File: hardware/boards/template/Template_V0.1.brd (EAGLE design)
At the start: 44 x 44 mm, 2 parts

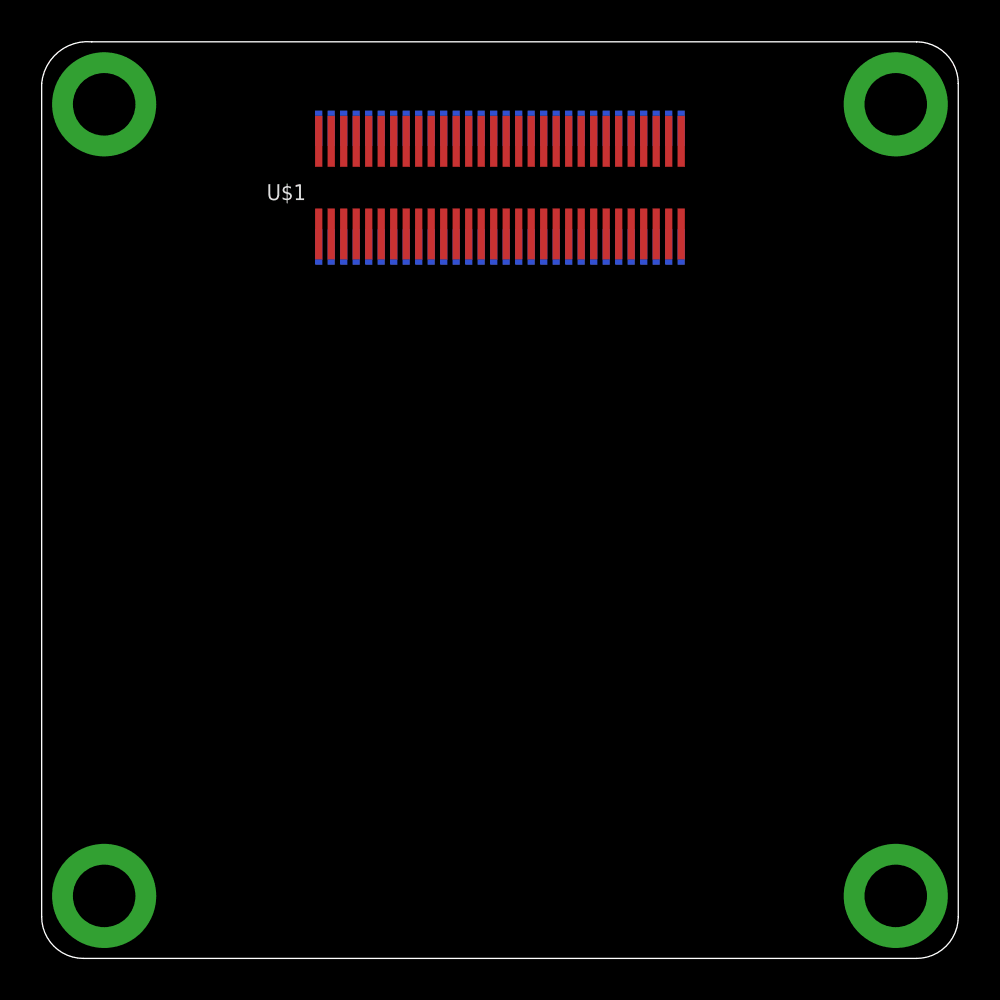
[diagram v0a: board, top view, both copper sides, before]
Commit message: Updating template, wip
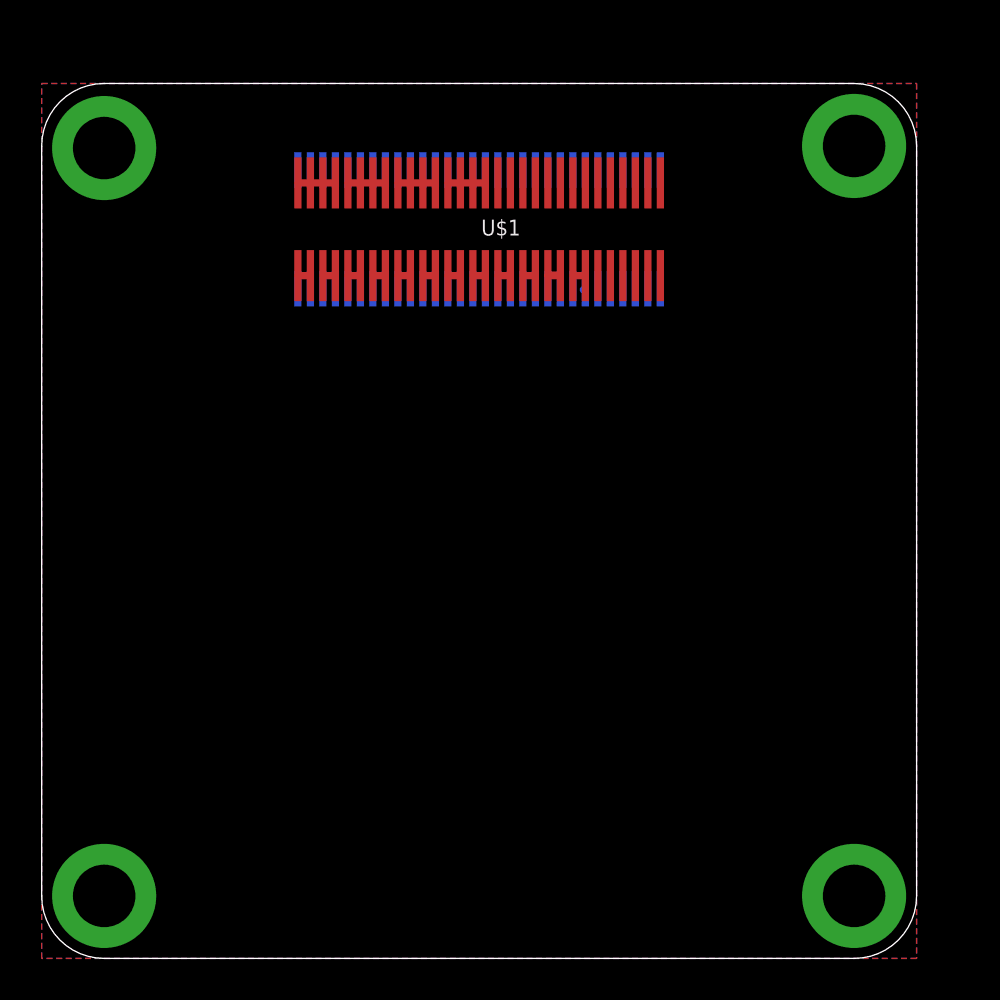
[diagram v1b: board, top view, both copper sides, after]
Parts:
- moved U$1 2.24 mm to (21.0, 35.0)
- moved U$3 2.24 mm to (21.0, 35.0)
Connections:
- removed net +3.3V_SW2: U$1.P$10, U$3.P$51
- removed net +3.3V_SW3: U$1.P$11, U$3.P$50
- removed net VBUS_1: U$1.P$53
- removed net VBUS_2: U$1.P$54
- removed net VBUS_3: U$1.P$55
- removed net VBUS_SW1: U$1.P$6, U$3.P$55
- removed net VBUS_SW2: U$1.P$7, U$3.P$54
- removed net VBUS_SW3: U$1.P$8, U$3.P$53
- new net +3V3_BUS: U$1.P$57, U$1.P$58, U$1.P$59, U$1.P$60
- new net +3V3_SW2: U$1.P$5, U$1.P$6, U$3.P$55, U$3.P$56
- new net +3V3_SW3: U$1.P$10, U$1.P$9, U$3.P$51, U$3.P$52
- new net /RST: U$1.P$27, U$3.P$34
- new net /SS/GPIO2: U$1.P$34
- new net 33-GND: U$3.P$3
- new net 37-GND: U$3.P$7
- new net 41-GND: U$3.P$11
- new net 44-GND: U$3.P$14
- new net 46-GND: U$3.P$16
- new net 48-GND: U$3.P$18
- new net 49-GND: U$3.P$19
- new net 57-GND: U$3.P$27
- new net 59-GND: U$3.P$29
- new net BATV_BUS: U$1.P$49, U$1.P$50, U$1.P$51, U$1.P$52
- new net BATV_SW1: U$1.P$13, U$1.P$14, U$3.P$47, U$3.P$48
- new net BATV_SW2: U$1.P$17, U$1.P$18, U$3.P$43, U$3.P$44
- new net BATV_SW3: U$1.P$21, U$1.P$22, U$3.P$39, U$3.P$40
- new net GPIO0: U$1.P$25, U$3.P$36
- new net GPIO1: U$1.P$26, U$3.P$35
- new net GPIO11: U$1.P$43
- new net GPIO12: U$1.P$44
- new net GPIO3: U$1.P$35
- new net GPIO4: U$1.P$36
- new net GPIO5: U$1.P$37
- new net GPIO6: U$1.P$38
- new net GPIO7: U$1.P$39
- new net GPIO8: U$1.P$40
- new net GPIO9: U$1.P$41
- new net MISO: U$1.P$32
- new net MOSI: U$1.P$31
- new net RTN_+3V3: U$1.P$53, U$1.P$54, U$1.P$55, U$1.P$56
- new net RTN_+3V3_SW1: U$1.P$3, U$1.P$4, U$3.P$57, U$3.P$58
- new net RTN_+3V3_SW2: U$1.P$7, U$1.P$8, U$3.P$53, U$3.P$54
- new net RTN_+3V3_SW3: U$1.P$11, U$1.P$12, U$3.P$49, U$3.P$50
- new net RTN_BATV: U$1.P$45, U$1.P$46, U$1.P$47, U$1.P$48
- new net RTN_BATV_SW1: U$1.P$15, U$1.P$16, U$3.P$45, U$3.P$46
- new net RTN_BATV_SW2: U$1.P$19, U$1.P$20, U$3.P$41, U$3.P$42
- new net RTN_BATV_SW3: U$1.P$23, U$1.P$24, U$3.P$37, U$3.P$38
- new net SCK: U$1.P$33
- new net SCL: U$1.P$29, U$3.P$32
- new net SDA: U$1.P$30, U$3.P$31
- net +3.3V_1: no longer U$1.P$50
- net +3.3V_2: no longer U$1.P$51
- net +3.3V_3: no longer U$1.P$52
- net +3.3V_SW1: now also U$1.P$1, U$1.P$2, U$3.P$59, U$3.P$60; no longer U$1.P$9, U$3.P$52
- net GND: now also U$1.P$28, U$3.P$33; no longer U$1.P$1, U$1.P$12, U$1.P$14, U$1.P$16, U$1.P$18, U$1.P$22, U$1.P$26, U$1.P$3, U$1.P$30, U$1.P$33, U$1.P$37, U$1.P$41, U$1.P$44, U$1.P$46, U$1.P$48, U$1.P$49, U$1.P$5, U$1.P$57, U$1.P$59, U$3.P$11, U$3.P$14, U$3.P$16, U$3.P$18, U$3.P$19, U$3.P$27, U$3.P$29, U$3.P$3, U$3.P$31, U$3.P$35, U$3.P$39, U$3.P$43, U$3.P$45, U$3.P$47, U$3.P$49, U$3.P$56, U$3.P$58, U$3.P$60, U$3.P$7
- net GPIO10: now also U$1.P$42; no longer U$1.P$31
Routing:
- net RTN_BATV: track 0.00 -> 1.80 mm
- net RTN_+3V3: track 0.00 -> 1.80 mm
- net +3V3_BUS: track 0.00 -> 1.80 mm
- net BATV_BUS: track 0.00 -> 1.80 mm
- net BATV_SW3: track 0.00 -> 1.11 mm
- net RTN_BATV_SW3: track 0.00 -> 0.72 mm
- net RTN_BATV_SW1: track 0.00 -> 0.60 mm
- net BATV_SW2: track 0.00 -> 0.60 mm
- net BATV_SW1: track 0.00 -> 0.60 mm
- net +3V3_SW2: track 0.00 -> 0.60 mm
- net RTN_+3V3_SW2: track 0.00 -> 0.60 mm
- net RTN_+3V3_SW1: track 0.00 -> 0.60 mm
- net +3.3V_SW1: track 0.00 -> 0.60 mm
- net RTN_BATV_SW2: track 0.00 -> 0.60 mm
- net RTN_+3V3_SW3: track 0.00 -> 0.60 mm
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- added copper zone on layer 1, net GND
- added copper zone on layer 16, net N$1
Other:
- board size 44 x 44 mm -> 42 x 42 mm
